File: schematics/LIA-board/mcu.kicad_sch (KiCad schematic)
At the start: 1 part, among them U2 STM32U575RGTx

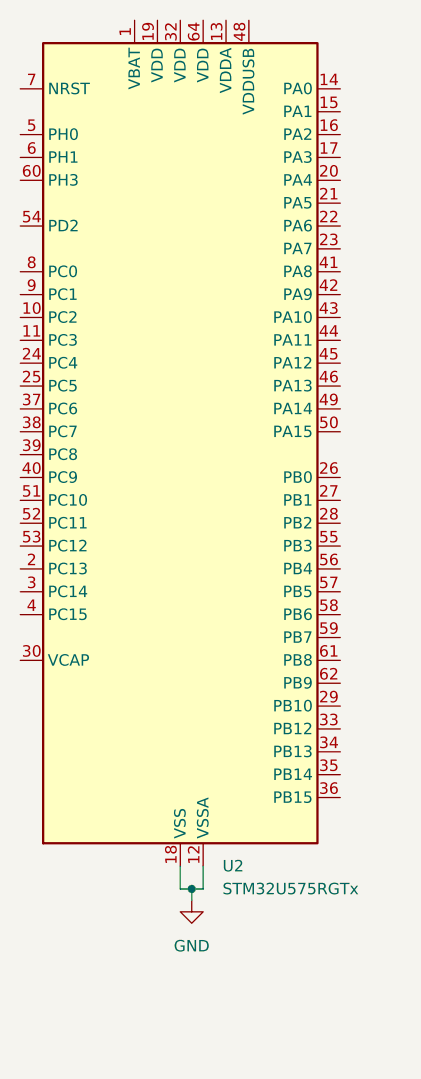
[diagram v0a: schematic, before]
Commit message: modified scematic
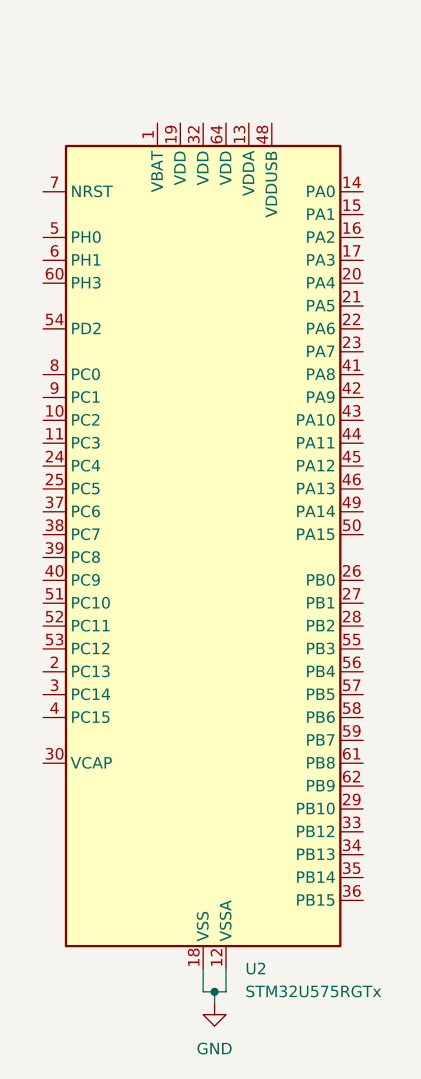
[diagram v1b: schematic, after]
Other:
- moved on the sheet: U2
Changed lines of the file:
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@@
 	(paper "A4")
 	(junction
-		(at 142.24 129.54)
+		(at 144.78 140.97)
 		(diameter 0)
 		(color 0 0 0 0)
@@
 	(wire
 		(pts
-			(xy 140.97 129.54) (xy 142.24 129.54)
-		)
-		(stroke
-			(width 0)
-			(type default)
-		)
-	)
-	(wire
-		(pts
-			(xy 142.24 129.54) (xy 142.24 130.81)
-		)
-		(stroke
-			(width 0)
-			(type default)
-		)
-	)
-	(wire
-		(pts
-			(xy 142.24 129.54) (xy 143.51 129.54)
-		)
-		(stroke
-			(width 0)
-			(type default)
-		)
-	)
-	(wire
-		(pts
-			(xy 140.97 127) (xy 140.97 129.54)
-		)
-		(stroke
-			(width 0)
-			(type default)
-		)
-	)
-	(wire
-		(pts
-			(xy 143.51 129.54) (xy 143.51 127)
+			(xy 143.51 140.97) (xy 144.78 140.97)
+		)
+		(stroke
+			(width 0)
+			(type default)
+		)
+	)
+	(wire
+		(pts
+			(xy 144.78 140.97) (xy 144.78 142.24)
+		)
+		(stroke
+			(width 0)
+			(type default)
+		)
+	)
+	(wire
+		(pts
+			(xy 144.78 140.97) (xy 146.05 140.97)
+		)
+		(stroke
+			(width 0)
+			(type default)
+		)
+	)
+	(wire
+		(pts
+			(xy 143.51 138.43) (xy 143.51 140.97)
+		)
+		(stroke
+			(width 0)
+			(type default)
+		)
+	)
+	(wire
+		(pts
+			(xy 146.05 140.97) (xy 146.05 138.43)
 		)
 		(stroke
@@
 	(symbol
 		(lib_id "MCU_ST_STM32U5:STM32U575RGTx")
-		(at 140.97 81.28 0)
+		(at 143.51 92.71 0)
 		(unit 1)
 		(body_style 1)
@@
 		(fields_autoplaced yes)
 		(property "Reference" "U2"
-			(at 145.6533 127 0)
+			(at 148.1933 138.43 0)
 			(show_name no)
 			(do_not_autoplace no)
@@
 		)
 		(property "Value" "STM32U575RGTx"
-			(at 145.6533 129.54 0)
+			(at 148.1933 140.97 0)
 			(show_name no)
 			(do_not_autoplace no)
@@
 		)
 		(property "Footprint" "Package_QFP:LQFP-64_10x10mm_P0.5mm"
-			(at 125.73 124.46 0)
+			(at 128.27 135.89 0)
 			(hide yes)
 			(show_name no)
@@
 		)
 		(property "Datasheet" "https://www.st.com/resource/en/datasheet/stm32u575rg.pdf"
-			(at 140.97 81.28 0)
+			(at 143.51 92.71 0)
 			(hide yes)
 			(show_name no)
@@
 		)
 		(property "Description" "STMicroelectronics Arm Cortex-M33 MCU, 1024KB flash, 786KB RAM, 160 MHz, 1.71-3.6V, 51 GPIO, LQFP64"
-			(at 140.97 81.28 0)
+			(at 143.51 92.71 0)
 			(hide yes)
 			(show_name no)
@@
 	(symbol
 		(lib_id "power:GND")
-		(at 142.24 130.81 0)
+		(at 144.78 142.24 0)
 		(unit 1)
 		(body_style 1)
@@
 		(fields_autoplaced yes)
 		(property "Reference" "#PWR070"
-			(at 142.24 137.16 0)
+			(at 144.78 148.59 0)
 			(hide yes)
 			(show_name no)
@@
 		)
 		(property "Value" "GND"
-			(at 142.24 135.89 0)
+			(at 144.78 147.32 0)
 			(show_name no)
 			(do_not_autoplace no)
@@
 		)
 		(property "Footprint" ""
-			(at 142.24 130.81 0)
+			(at 144.78 142.24 0)
 			(hide yes)
 			(show_name no)
@@
 		)
 		(property "Datasheet" ""
-			(at 142.24 130.81 0)
+			(at 144.78 142.24 0)
 			(hide yes)
 			(show_name no)
@@
 		)
 		(property "Description" "Power symbol creates a global label with name \"GND\" , ground"
-			(at 142.24 130.81 0)
-			(hide yes)
-			(show_name no)
+			(at 144.78 142.24 0)
+			(hide yes)
+			(show_name no)
